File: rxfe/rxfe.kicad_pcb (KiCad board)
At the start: 2 copper layers, 129.3 x 45.7 mm, 85 parts, among them J1 SMA, J2 SMA, J3 4610X-AP1-103LF, J4 SMA, K1 CONN_3, P1 CONN_8X2, U1 SKY12347, U10 SMP1330-005LF, U11 LTC1983-5, U12 SMP1330-005LF, U13 LDO_78XX, U14 TCM809, U15 GALI-84+, U16 GALI-84+, U2 74HC04, U3 SCLF-25, U4 HMC595, U5 HMC595, U6 MAR-8ASM+, U7 SWMA-2-50DR+, U8 HMC595, U9 HMC595

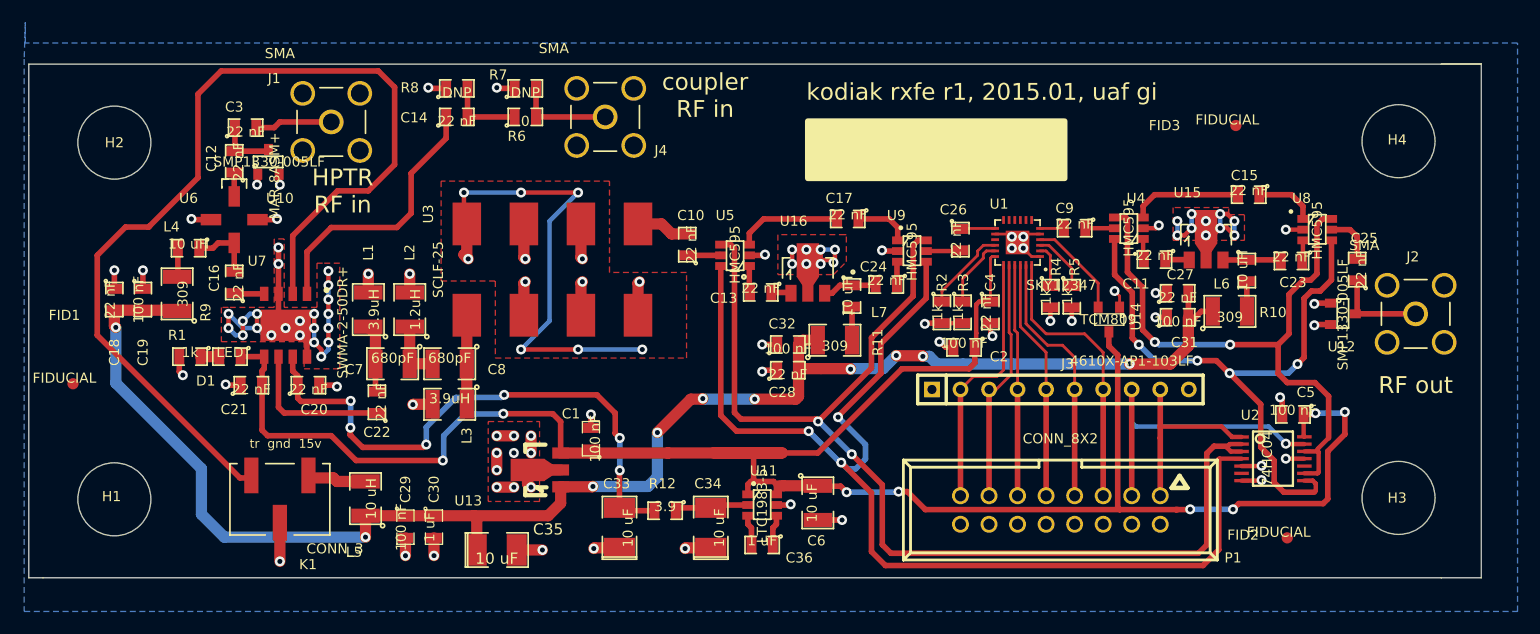
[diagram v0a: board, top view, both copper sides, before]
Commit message: DFM changes..
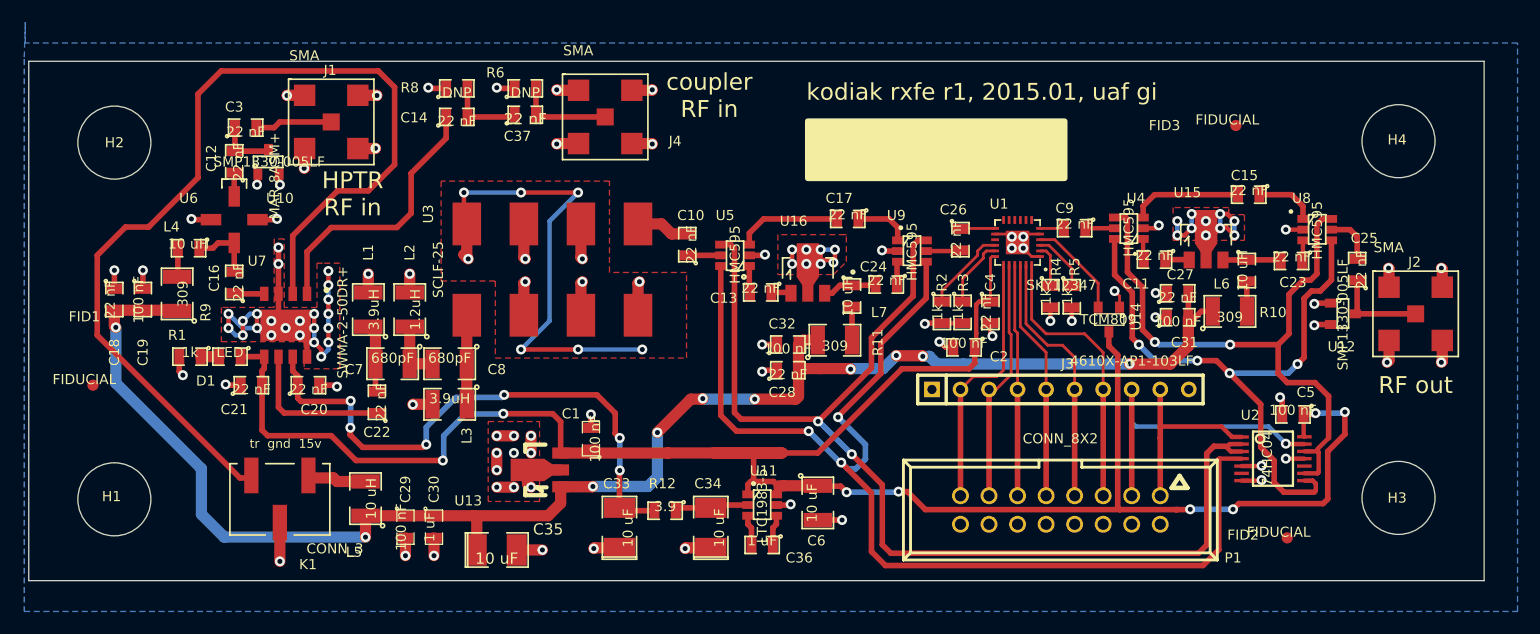
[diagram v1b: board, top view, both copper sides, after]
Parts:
- removed R7: 0, SMD_Packages:SMD-0805
- added C37: 22 nF, SMD_Packages:SMD-0805, F.Cu at (140.7, 87.1)
- J1, J2, J4: footprint local:SMA_5-1814832-1 -> local:SMA_0732511350
- moved FID1 1.78 mm to (102.2, 111.1)
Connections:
- net VCC renamed +5V
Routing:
- net GND: track 242.7 -> 267.0 mm, vias 109 -> 122
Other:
- board size 129.3 x 45.7 mm -> 129.5 x 46.2 mm
